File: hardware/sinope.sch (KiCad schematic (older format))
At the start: 52 parts, among them J1 PIOA, J2 SERIAL1, J3 PIOB, J4 USB_B_Micro, J7 Z80_BUS, Q1 MMBT3904, SW1 RESET, U1 Z80CPU, U10 MEMORY_GAL, U11 74LS157, U12 TC551001, U2 Z80CTC, U3 Z80PIO, U4 Z80SIO, U5 MAX232, U6 FT232RL, U7 IO_GAL, U8 MAX695, U9 27C010, X1 3.6864Mhz

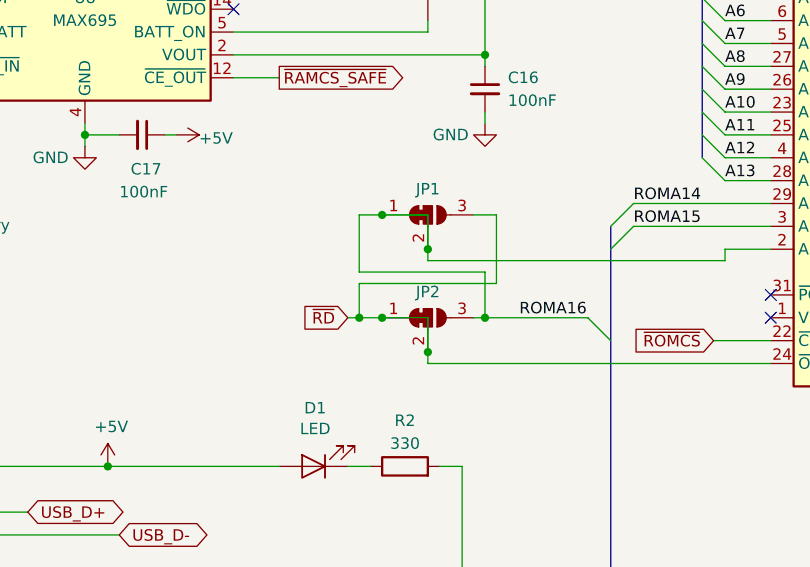
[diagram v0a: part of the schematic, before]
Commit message: Layout redone quickly
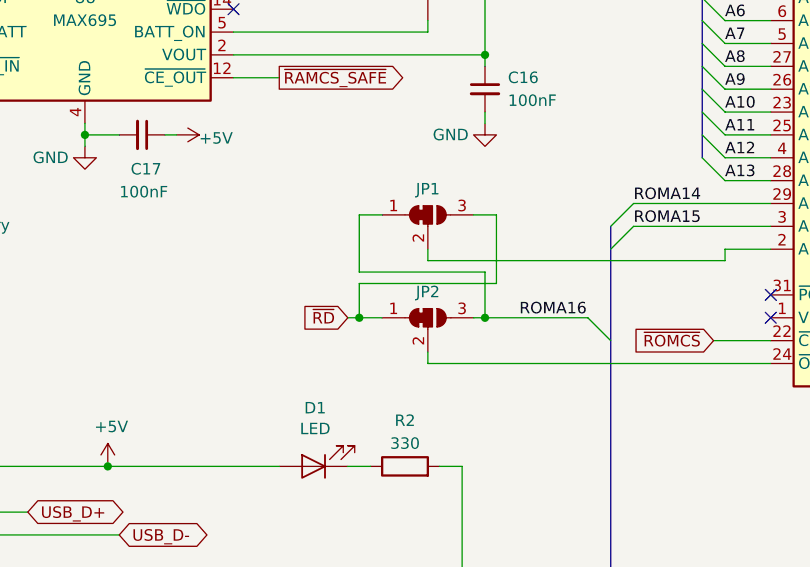
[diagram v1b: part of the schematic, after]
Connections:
- wire segments 521 -> 517
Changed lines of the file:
@@
 	6350 8650 6400 8650
 Connection ~ 6400 8650
-Wire Wire Line
-	5950 8200 6150 8200
-Wire Wire Line
-	6150 8200 6150 8350
-Connection ~ 5950 8200
-Connection ~ 6150 8350
-Wire Wire Line
-	5950 8650 6150 8650
-Wire Wire Line
-	6150 8650 6150 8800
 Wire Bus Line
 	6950 8250 6950 10250
@@
 Wire Bus Line
 	2700 6250 2700 7900
-Connection ~ 5950 8650
-Connection ~ 6150 8800
 $EndSCHEMATC
